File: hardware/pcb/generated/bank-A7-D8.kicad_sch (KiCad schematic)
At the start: 34 parts, among them U54 SK9822-EC20, U55 SK9822-EC20, U56 SK9822-EC20, U57 SK9822-EC20, U66 SK9822-EC20, U67 SK9822-EC20, U68 SK9822-EC20, U69 SK9822-EC20, U72 TCA9554DWR

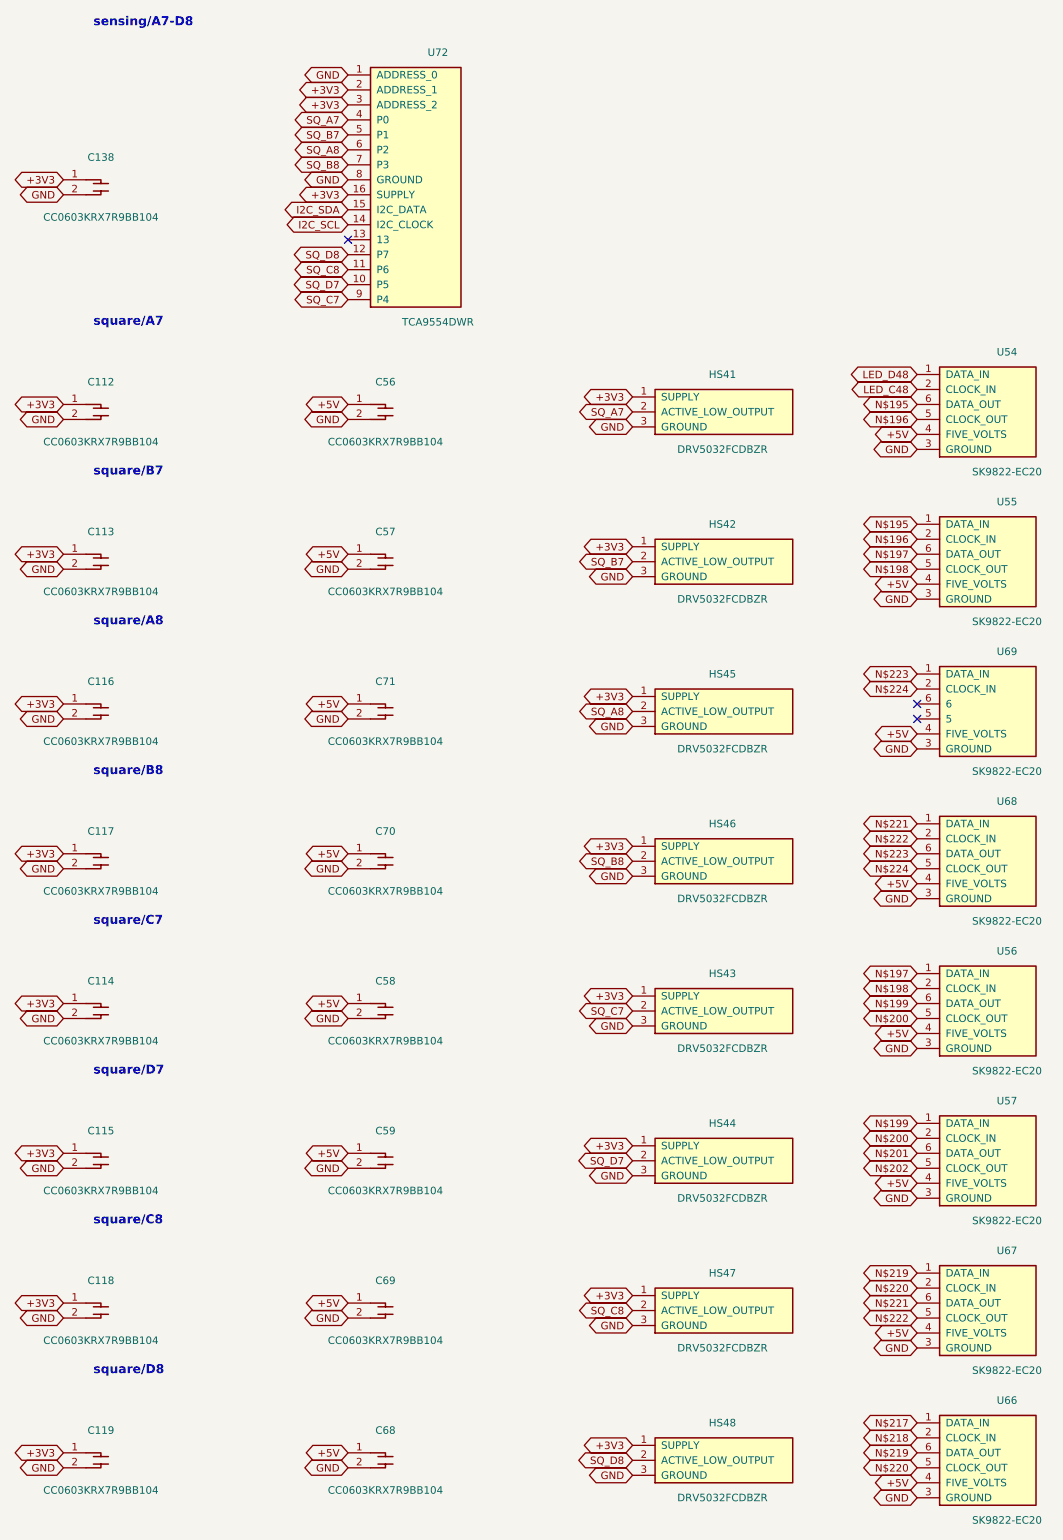
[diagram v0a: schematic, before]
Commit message: chore(pcb): regenerate KiCad, SPICE and review output
Generated by `just pcb` from the committed definition; not hand-edited.
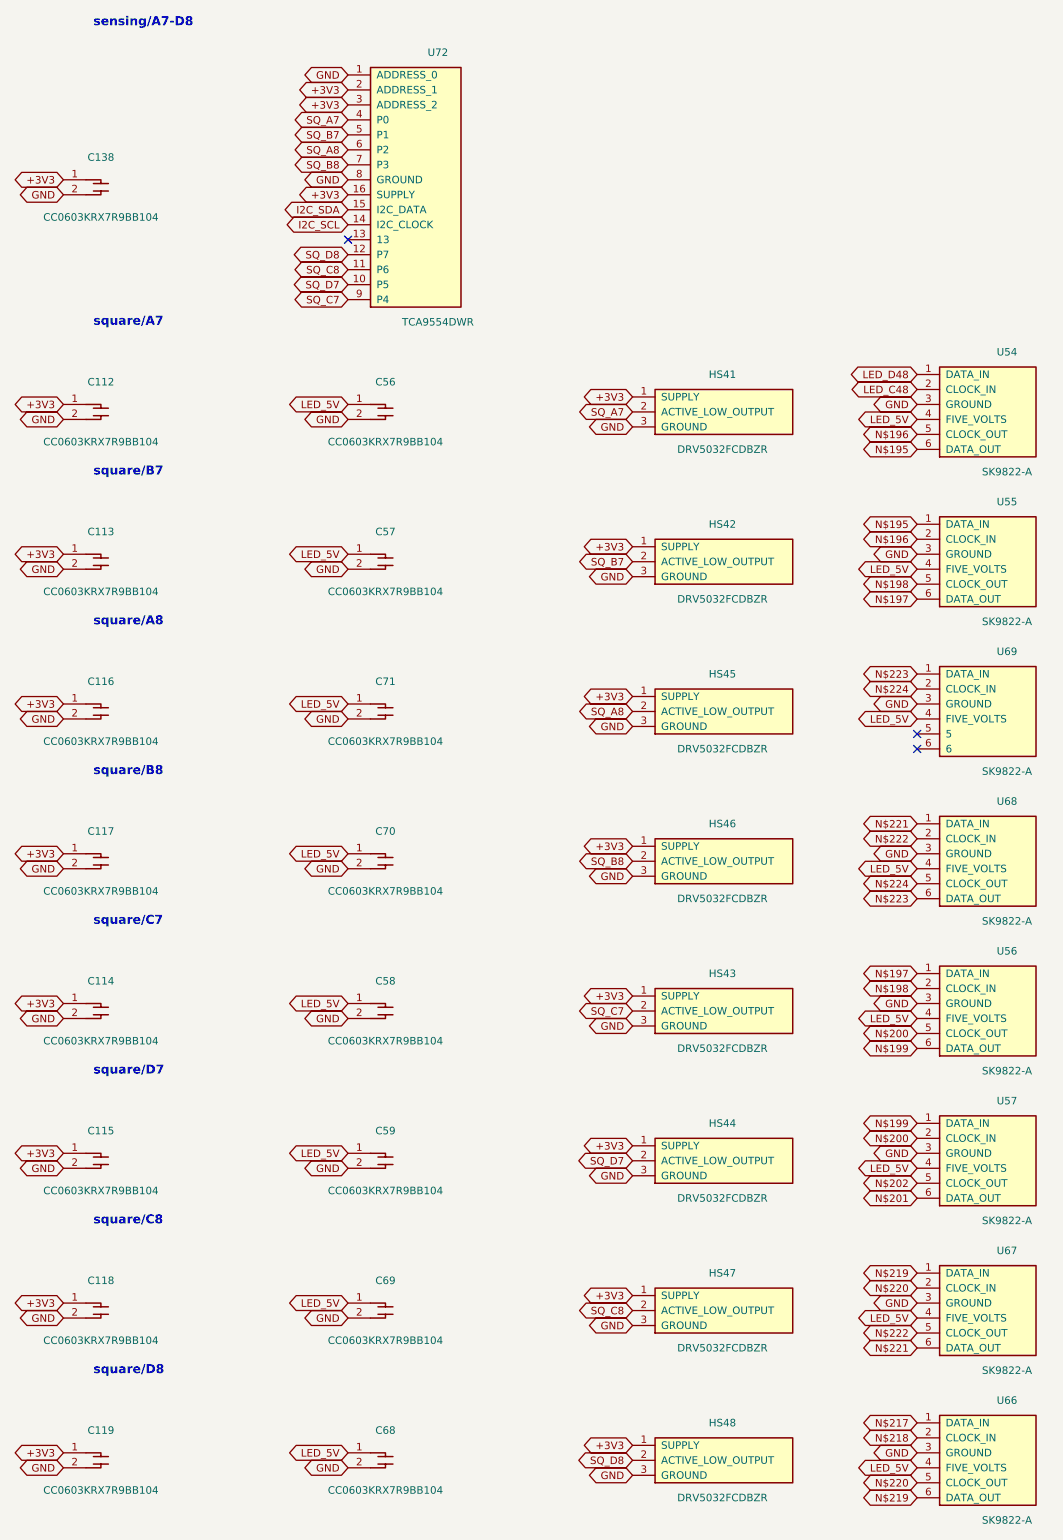
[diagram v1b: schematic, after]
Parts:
- U54, U55, U56, U57, U66, U67, U68, U69: value SK9822-EC20 -> SK9822-A
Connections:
- net +5V renamed LED_5V
